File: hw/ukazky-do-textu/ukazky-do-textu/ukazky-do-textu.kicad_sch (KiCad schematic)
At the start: 7 parts, among them J1 Konektor

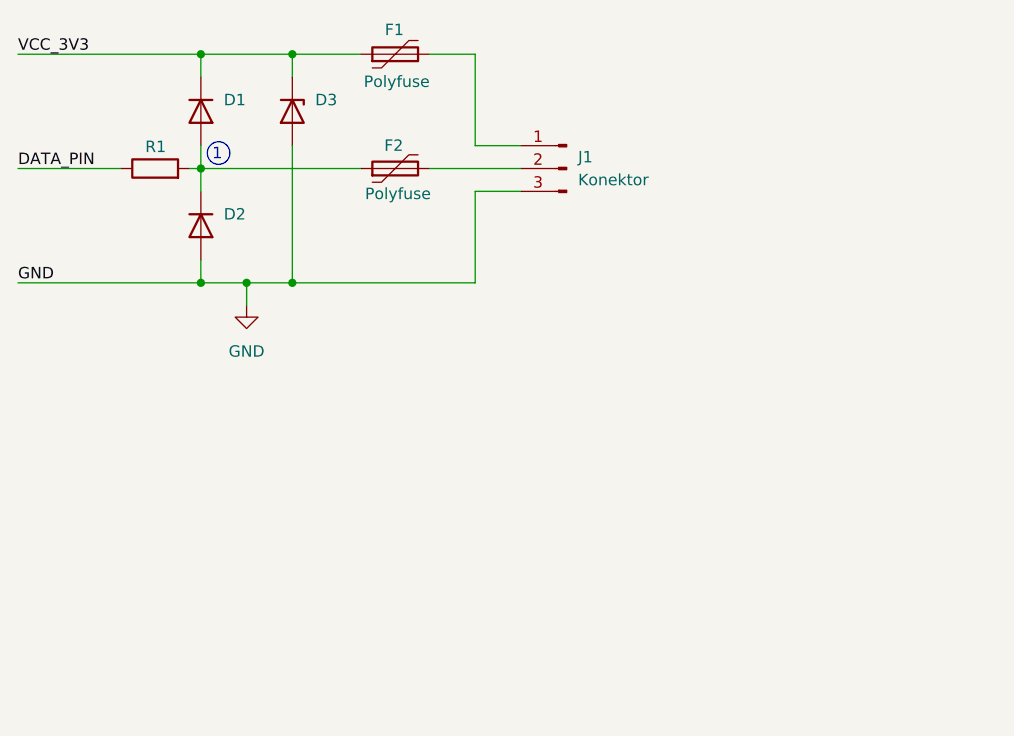
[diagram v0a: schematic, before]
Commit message: schemata a 3d modely pro text
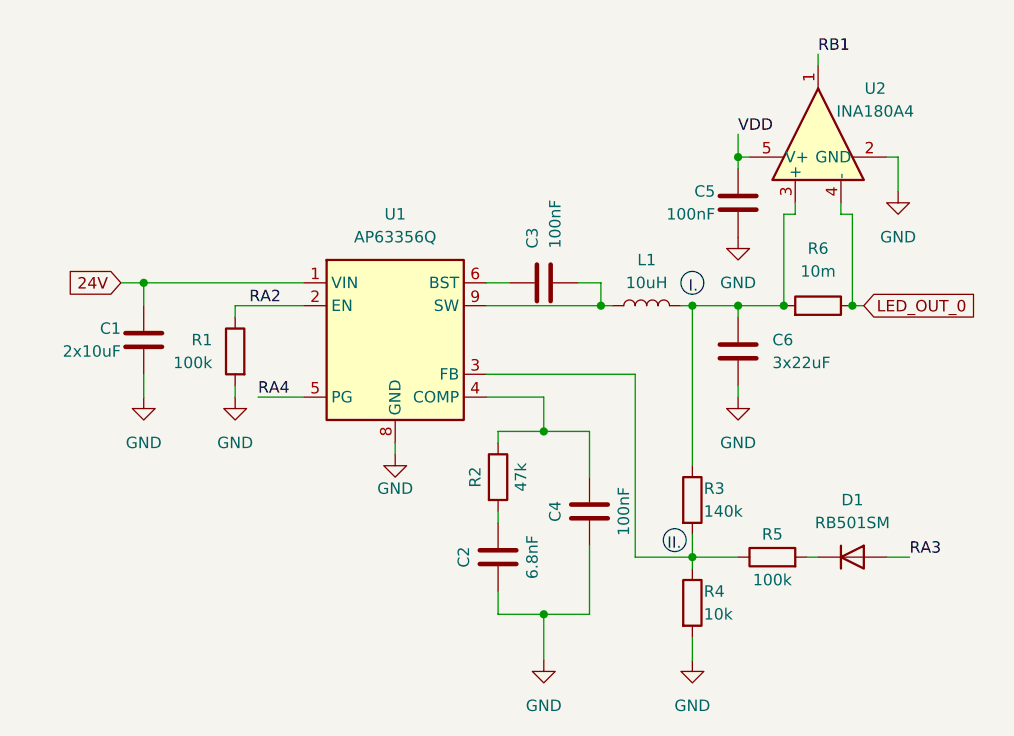
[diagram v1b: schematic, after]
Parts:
- removed D1, D2: 1N914, Diode_THT:D_DO-35_SOD27_P7.62mm_Horizontal, symbol Diode:1N914
- removed D3: D_Zener, symbol Device:D_Zener
- removed F1, F2: Polyfuse, symbol Device:Polyfuse
- removed J1: Konektor, symbol Connector:Conn_01x03_Pin
- added C1: 2x10uF, Capacitor_SMD:C_1210_3225Metric_Pad1.33x2.70mm_HandSolder, symbol Device:C
- added C2: 6.8nF, Capacitor_SMD:C_0805_2012Metric_Pad1.18x1.45mm_HandSolder, symbol Device:C
- added C3, C4, C5: 100nF, Capacitor_SMD:C_0805_2012Metric_Pad1.18x1.45mm_HandSolder, symbol Device:C
- added C6: 3x22uF, Capacitor_SMD:C_0805_2012Metric_Pad1.18x1.45mm_HandSolder, symbol Device:C
- added D1: RB501SM, Diode_SMD:D_SOD-523, symbol Device:D
- added L1: 10uH, Inductor_SMD:L_Changjiang_FNR6045S, symbol Device:L
- added R2: 47k, Resistor_SMD:R_0805_2012Metric_Pad1.20x1.40mm_HandSolder, symbol Device:R
- added R3: 140k, Resistor_SMD:R_0805_2012Metric_Pad1.20x1.40mm_HandSolder, symbol Device:R
- added R4: 10k, Resistor_SMD:R_0805_2012Metric_Pad1.20x1.40mm_HandSolder, symbol Device:R
- added R5: 100k, Resistor_SMD:R_0805_2012Metric_Pad1.20x1.40mm_HandSolder, symbol Device:R
- added R6: 10m, Resistor_SMD:R_0815_2038Metric_Pad1.20x4.05mm_HandSolder, symbol Device:R
- added U1: AP63356Q, Library:V-DFN3020-13, symbol buck-lib:AP63356Q
- added U2: INA180A4, Package_TO_SOT_SMD:SOT-23-5, symbol Amplifier_Current:INA180A4
- R1: value R -> 100k; footprint (none) -> Resistor_SMD:R_0805_2012Metric_Pad1.20x1.40mm_HandSolder
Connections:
- net GND: now also R1.2, C1.2, C2.1, C4.1, C5.2, C6.2, R4.2, U1.8 (GND), U2.2 (GND)
- net DATA_PIN renamed RA2
- net RA2: now also U1.2 (EN)
- new net: C6.1, L1.1, R3.1, R6.2, U2.3 (+)
- new net: C3.2, L1.2, U1.9 (SW)
- new net: R3.2, R4.1, R5.1, U1.3 (FB)
- new net: D1.1 (K), R5.2
- new net: C4.2, R2.1, U1.4 (COMP)
- new net: C2.2, R2.2
- new net: C3.1, U1.6 (BST)
- new net 24V: C1.1, U1.1 (VIN)
- new net LED_OUT_0: R6.1, U2.4 (-)
- new net RA3: D1.2 (A)
- new net RA4: U1.5 (PG)
- new net RB1: U2.1
- new net VDD: C5.1, U2.5 (V+)
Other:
- note added: "I."
- note added: "II."
- note removed: "1"
